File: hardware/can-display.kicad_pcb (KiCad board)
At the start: 4 copper layers, 35.6 x 29.2 mm, 30 parts, among them J1 Conn_01x10_Female, J2 Conn_02x09_Odd_Even, J3 Conn_01x04_Male, J4 Conn_01x02_Male, J5 Conn_01x04_Male, J6 Conn_01x04_Male, U1 STM32F072C8Tx, U2 MCP4019, U3 TLC59284, U4 MCP2562, U5 L7805, U6 AP2204K-3.3, U7 MIC4427

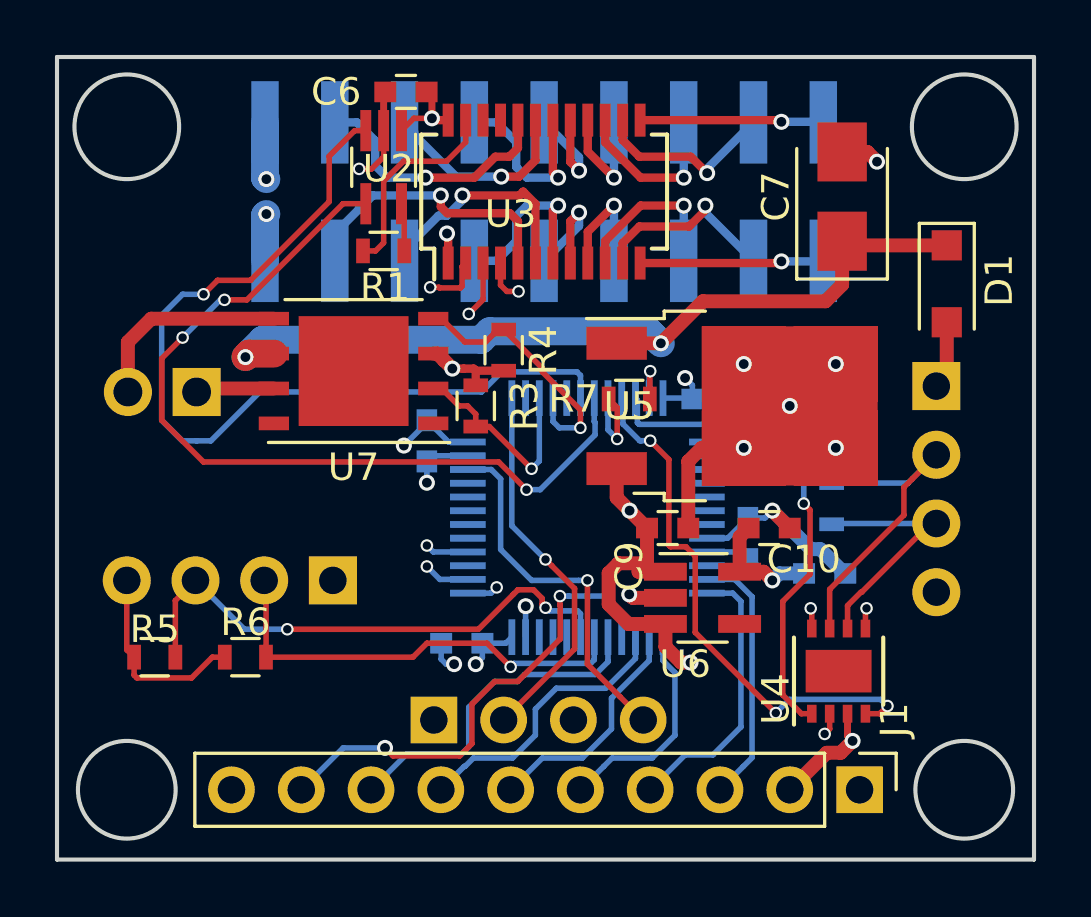
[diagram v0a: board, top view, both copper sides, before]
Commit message: schematic and route f4
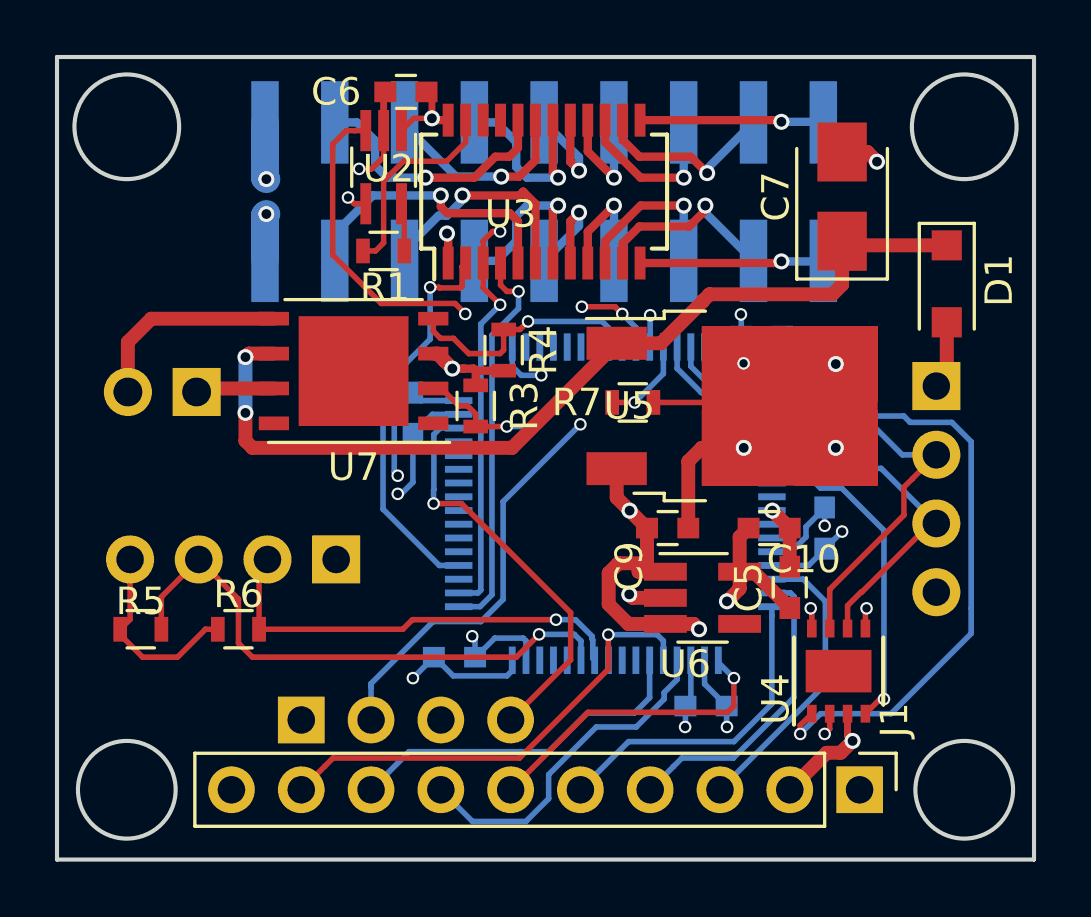
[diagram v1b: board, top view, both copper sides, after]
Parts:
- added C8: 0.1uF, Capacitors_SMD:C_0603, B.Cu at (49.0, 49.0)
- C5: moved to F.Cu
- U1: value STM32F072C8Tx -> STM32F446RCTx; footprint Housings_QFP:LQFP-48_7x7mm_Pitch0.5mm -> Housings_QFP:LQFP-64_10x10mm_Pitch0.5mm
- moved J6 4.83 mm to (34.3, 49.5)
- moved C3 2.90 mm to (51.1, 35.6)
- moved C2 2.82 mm to (53.3, 42.5)
- moved R2 2.04 mm to (53.7, 39.6)
- moved C5 1.37 mm to (52.1, 44.7), turned to 90 degrees
- moved U1 1.14 mm to (45.7, 41.7)
- moved R5 1.14 mm to (28.4, 46.2)
- moved C4 1.13 mm to (38.4, 38.4)
- moved R6 1.05 mm to (32.0, 46.2)
- moved J5 0.77 mm to (35.6, 43.7)
- moved C1 0.57 mm to (39.9, 47.2), turned to 0 degrees
- moved R7 0.18 mm to (46.4, 38.0)
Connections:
- U1 pad 11: OLED_SDCS -> (no net)
- U1 pad 12: OLED_OCS -> GND
- U1 pad 13: OLED_RST -> +3V3
- U1 pad 14: OLED_DC -> OLED_SDCS
- U1 pad 15: OLED_SCK -> OLED_OCS
- U1 pad 16: OLED_MISO -> OLED_RST
- U1 pad 17: OLED_MOSI -> OLED_DC
- U1 pad 18: ADC_KNOB -> GND
- U1 pad 19: ADC_KNOB2 -> +3V3
- U1 pad 20: (no net) -> OLED_SCK
- U1 pad 21: (no net) -> OLED_MISO
- U1 pad 22: (no net) -> OLED_MOSI
- U1 pad 23: GND -> (no net)
- U1 pad 24: +3V3 -> (no net)
- U1 pad 25: LED_LAT -> (no net)
- U1 pad 26: LED_SCK -> ADC_KNOB
- U1 pad 27: (no net) -> ADC_KNOB2
- U1 pad 28: LED_MOSI -> (no net)
- U1 pad 31: (no net) -> GND
- U1 pad 32: (no net) -> +3V3
- U1 pad 33: (no net) -> LED_LAT
- U1 pad 34: Net-(J6-Pad4) -> LED_SCK
- U1 pad 35: GND -> (no net)
- U1 pad 36: +3V3 -> LED_MOSI
- U1 pad 37: Net-(J6-Pad2) -> (no net)
- U1 pad 39: DRIVER_1 -> (no net)
- U1 pad 40: DRIVER_2 -> (no net)
- U1 pad 42: SCL -> (no net)
- U1 pad 43: SDA -> (no net)
- U1 pad 44: Net-(R7-Pad1) -> (no net)
- U1 pad 45: CAN_RX -> (no net)
- U1 pad 46: CAN_TX -> Net-(J6-Pad4)
- U1 pad 8: GND -> (no net)
- U1 pad 9: +3V3 -> (no net)
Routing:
- net SDA: track 31.0 -> 15.4 mm, vias 3 -> 2
- net SCL: track 32.8 -> 18.7 mm, vias 1 -> 3
- net CAN_TX: track 18.1 -> 27.9 mm
- net +3V3: track 17.9 -> 26.3 mm, vias 6 -> 8
- net GND: track 48.2 -> 56.4 mm, vias 17 -> 16
- net Net-(J6-Pad2): track 13.7 -> 19.2 mm, vias 1 -> 2
- net OLED_RST: track 8.01 -> 12.4 mm
- net OLED_DC: track 8.50 -> 11.7 mm, vias 0 -> 1
- net +12V: track 31.3 -> 33.9 mm
- net OLED_SCK: track 10.4 -> 12.6 mm
- net Net-(J6-Pad4): track 13.4 -> 15.0 mm
- net OLED_SDCS: track 9.42 -> 10.7 mm
- net OLED_OCS: track 10.2 -> 11.2 mm
- net LED_SCK: track 14.1 -> 14.9 mm
- net ADC_KNOB2: track 19.8 -> 20.6 mm, vias 2 -> 1
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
